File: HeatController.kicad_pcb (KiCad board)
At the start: 2 copper layers, 75.7 x 65.8 mm, 70 parts, among them J1 Screw_Terminal_01x02, J2 Screw_Terminal_01x02, J3 Screw_Terminal_01x02, J4 Screw_Terminal_01x02, J5 Screw_Terminal_01x02, J6 Screw_Terminal_01x02, Q1 IRF3205, Q2 IRF3205, Q3 IRF3205, Q4 IRF3205, Q5 IRF3205, Q6 IRF3205, U1 WeMos_D1_mini, U2 LMR14010ADDC

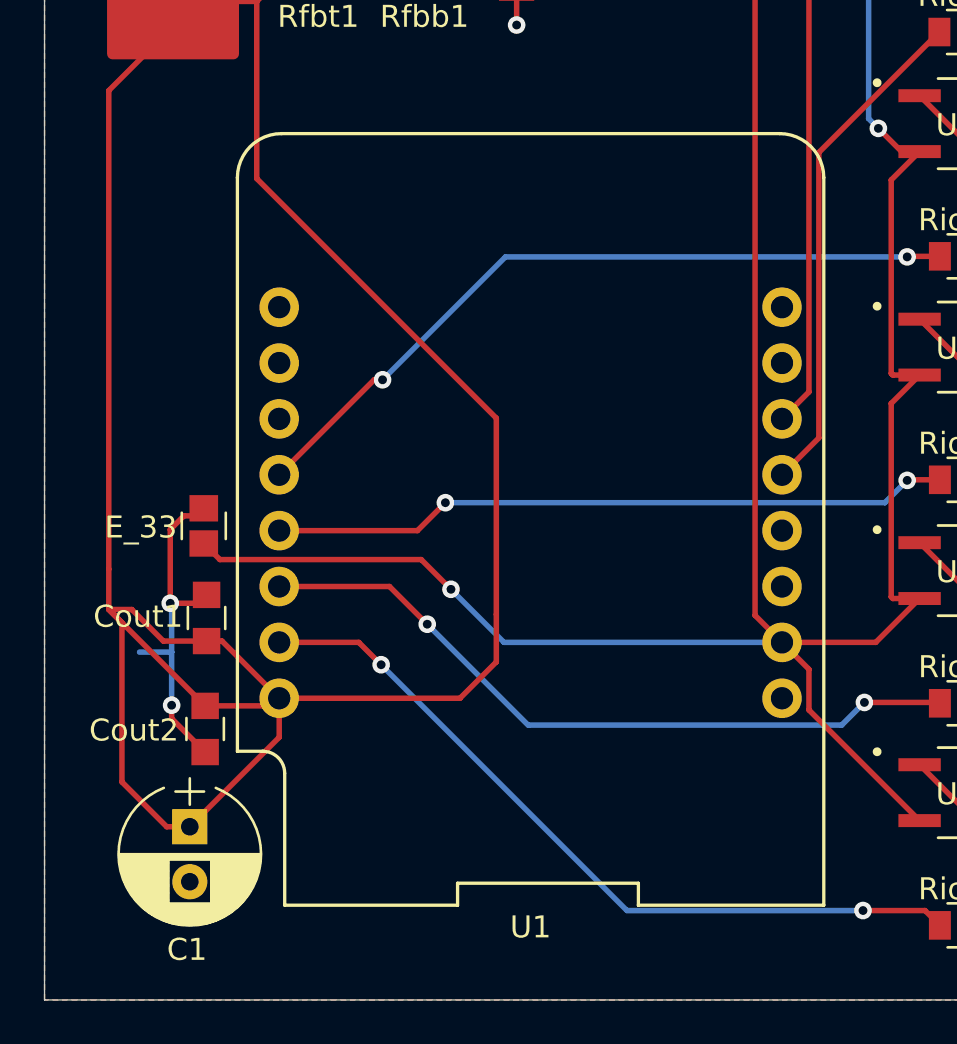
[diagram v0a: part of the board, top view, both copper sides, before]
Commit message: backup lenovo
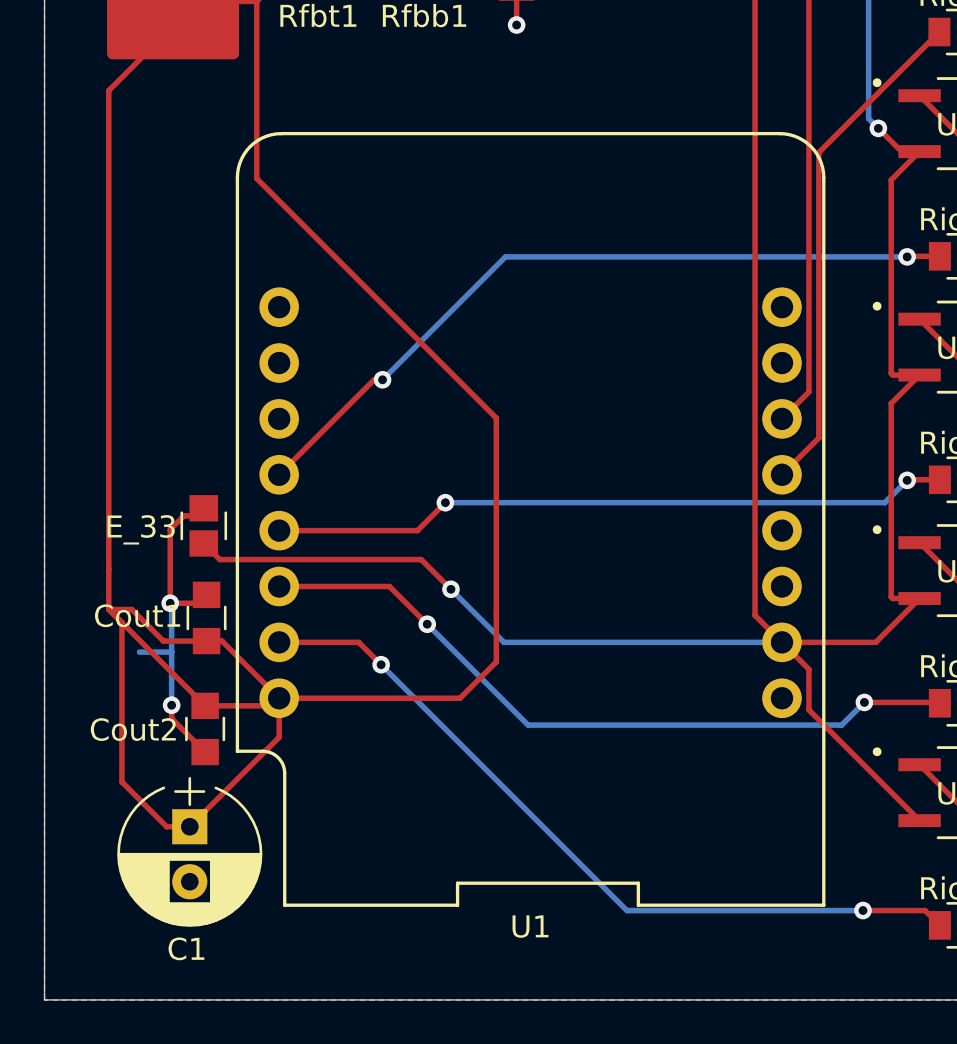
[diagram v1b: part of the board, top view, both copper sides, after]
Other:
- net class Default removed
